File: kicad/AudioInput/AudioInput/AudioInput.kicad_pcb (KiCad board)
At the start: 2 copper layers, 48.9 x 55.5 mm, 61 parts, among them J1 EXPAN2, J2 EXPAN1, J3 INT INPUT, K1 G6K-2, Q1 BS250, Q2 2N7000, Q3 BS250, U1 MCP4651, U2 LM324, U3 CD4052B

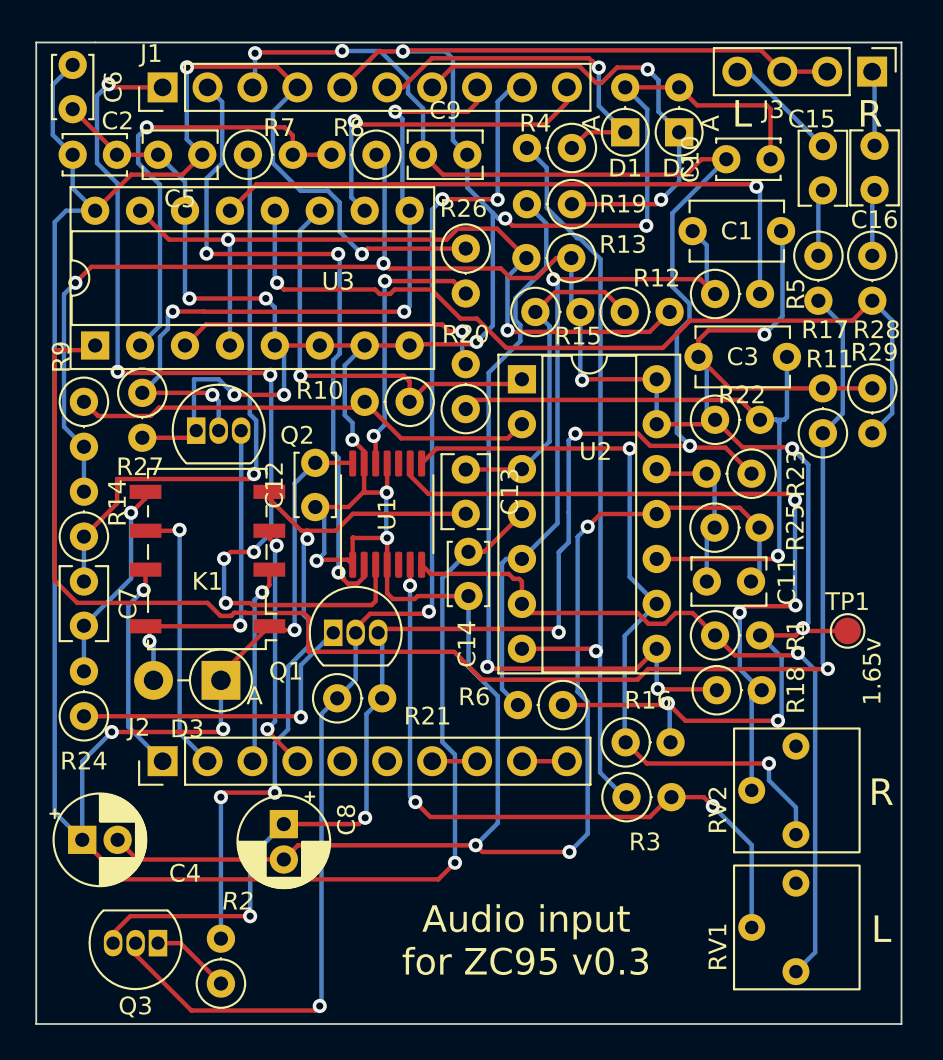
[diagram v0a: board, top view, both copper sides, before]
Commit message: Audio input board v0.4
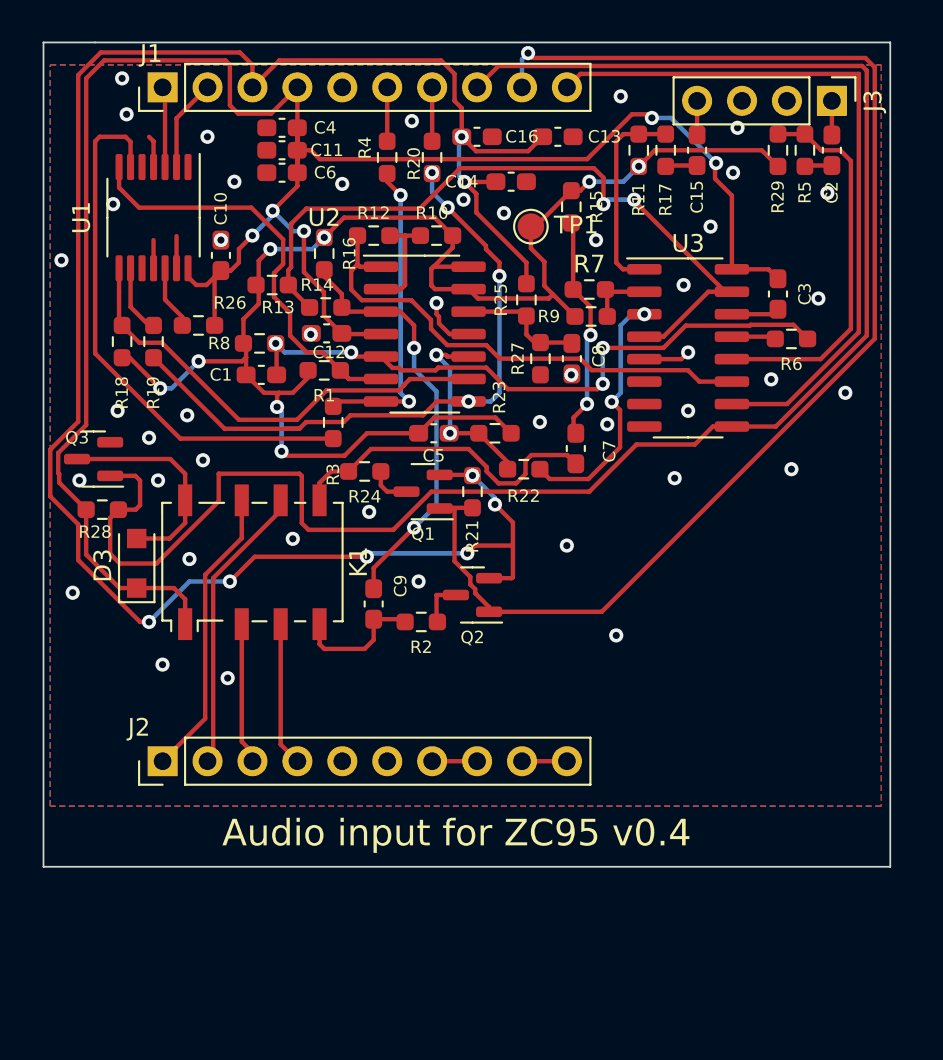
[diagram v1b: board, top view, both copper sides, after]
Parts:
- removed D1, D2: 3.3v, Diode_THT:D_DO-35_SOD27_P2.54mm_Vertical_AnodeUp
- removed RV1, RV2: 50k, Library:3362P-1-503
- C1: value 3nF -> 3.3nF; footprint Capacitor_THT:C_Disc_D5.1mm_W3.2mm_P5.00mm -> Capacitor_SMD:C_0603_1608Metric_Pad1.08x0.95mm_HandSolder
- C10, C12, C6: footprint Capacitor_THT:C_Disc_D3.4mm_W2.1mm_P2.50mm -> Capacitor_SMD:C_0603_1608Metric_Pad1.08x0.95mm_HandSolder
- C11, C15, C7, C9: footprint Capacitor_THT:C_Rect_L4.0mm_W2.5mm_P2.50mm -> Capacitor_SMD:C_0603_1608Metric_Pad1.08x0.95mm_HandSolder
- C13: value 1uF -> 10uF; footprint Capacitor_THT:C_Rect_L4.0mm_W2.5mm_P2.50mm -> Capacitor_SMD:C_0603_1608Metric_Pad1.08x0.95mm_HandSolder
- C14, C2: value 100nF -> 1uF; footprint Capacitor_THT:C_Disc_D3.4mm_W2.1mm_P2.50mm -> Capacitor_SMD:C_0603_1608Metric_Pad1.08x0.95mm_HandSolder
- C16: value 1uF -> 100nF; footprint Capacitor_THT:C_Rect_L4.0mm_W2.5mm_P2.50mm -> Capacitor_SMD:C_0603_1608Metric_Pad1.08x0.95mm_HandSolder
- C3: value 3nF -> 100nF; footprint Capacitor_THT:C_Disc_D5.1mm_W3.2mm_P5.00mm -> Capacitor_SMD:C_0603_1608Metric_Pad1.08x0.95mm_HandSolder
- C4: footprint Capacitor_THT:CP_Radial_D5.0mm_P2.00mm -> Capacitor_SMD:C_0603_1608Metric_Pad1.08x0.95mm_HandSolder
- C5: value 1uF -> 3.3nF; footprint Capacitor_THT:C_Rect_L4.0mm_W2.5mm_P2.50mm -> Capacitor_SMD:C_0603_1608Metric_Pad1.08x0.95mm_HandSolder
- C8: value 10uF -> 1uF; footprint Capacitor_THT:CP_Radial_D5.0mm_P2.00mm -> Capacitor_SMD:C_0603_1608Metric_Pad1.08x0.95mm_HandSolder
- D3: value 1N4004 -> SM4007PL; footprint Diode_THT:D_DO-41_SOD81_P3.81mm_Vertical_AnodeUp -> Diode_SMD:D_SOD-123F
- Q1: value BS250 -> AO3401A; footprint Package_TO_SOT_THT:TO-92_Inline -> Package_TO_SOT_SMD:SOT-23
- Q2: value 2N7000 -> AO3401A; footprint Package_TO_SOT_THT:TO-92_Inline -> Package_TO_SOT_SMD:SOT-23
- Q3: value BS250 -> AO3400A; footprint Package_TO_SOT_THT:TO-92_Inline -> Package_TO_SOT_SMD:SOT-23
- R1, R11, R12, R15, R17, R21, R23, R25, R26, R27, R28, R29, R3, R4, R7: footprint Resistor_THT:R_Axial_DIN0207_L6.3mm_D2.5mm_P2.54mm_Vertical -> Resistor_SMD:R_0603_1608Metric_Pad0.98x0.95mm_HandSolder
- R10: value 100k -> 4k7; footprint Resistor_THT:R_Axial_DIN0207_L6.3mm_D2.5mm_P2.54mm_Vertical -> Resistor_SMD:R_0603_1608Metric_Pad0.98x0.95mm_HandSolder
- R13, R8: value 150k -> 100k; footprint Resistor_THT:R_Axial_DIN0207_L6.3mm_D2.5mm_P2.54mm_Vertical -> Resistor_SMD:R_0603_1608Metric_Pad0.98x0.95mm_HandSolder
- R14: value 100k -> 150k; footprint Resistor_THT:R_Axial_DIN0207_L6.3mm_D2.5mm_P2.54mm_Vertical -> Resistor_SMD:R_0603_1608Metric_Pad0.98x0.95mm_HandSolder
- R16: value 4k7 -> 100k; footprint Resistor_THT:R_Axial_DIN0207_L6.3mm_D2.5mm_P2.54mm_Vertical -> Resistor_SMD:R_0603_1608Metric_Pad0.98x0.95mm_HandSolder
- R18: value 10k -> 4k7; footprint Resistor_THT:R_Axial_DIN0207_L6.3mm_D2.5mm_P2.54mm_Vertical -> Resistor_SMD:R_0603_1608Metric_Pad0.98x0.95mm_HandSolder
- R19: value 1k -> 10k; footprint Resistor_THT:R_Axial_DIN0207_L6.3mm_D2.5mm_P2.54mm_Vertical -> Resistor_SMD:R_0603_1608Metric_Pad0.98x0.95mm_HandSolder
- R2, R24: value 2k7 -> 2k2; footprint Resistor_THT:R_Axial_DIN0207_L6.3mm_D2.5mm_P2.54mm_Vertical -> Resistor_SMD:R_0603_1608Metric_Pad0.98x0.95mm_HandSolder
- R20: value 10k -> 1k; footprint Resistor_THT:R_Axial_DIN0207_L6.3mm_D2.5mm_P2.54mm_Vertical -> Resistor_SMD:R_0603_1608Metric_Pad0.98x0.95mm_HandSolder
- R22, R6: value 100k -> 10k; footprint Resistor_THT:R_Axial_DIN0207_L6.3mm_D2.5mm_P2.54mm_Vertical -> Resistor_SMD:R_0603_1608Metric_Pad0.98x0.95mm_HandSolder
- R5: value 10k -> 100k; footprint Resistor_THT:R_Axial_DIN0207_L6.3mm_D2.5mm_P2.54mm_Vertical -> Resistor_SMD:R_0603_1608Metric_Pad0.98x0.95mm_HandSolder
- R9: value 10k -> 150k; footprint Resistor_THT:R_Axial_DIN0207_L6.3mm_D2.5mm_P2.54mm_Vertical -> Resistor_SMD:R_0603_1608Metric_Pad0.98x0.95mm_HandSolder
- U2: footprint Package_DIP:DIP-14_W7.62mm_Socket -> Package_SO:SOIC-14_3.9x8.7mm_P1.27mm
- U3: footprint Package_DIP:DIP-16_W7.62mm_Socket -> Package_SO:SOIC-16_3.9x9.9mm_P1.27mm
- moved R28 45.8 mm to (132.5, 89.9), turned to 0 degrees
- moved C4 41.8 mm to (142.6, 68.3), turned to 180 degrees
- moved C2 40.4 mm to (173.7, 69.6), turned to -90 degrees
- moved R18 39.0 mm to (133.6, 80.4), turned to -90 degrees
- moved C11 36.0 mm to (142.6, 69.6), turned to 0 degrees
- moved U3 33.5 mm to (165.6, 80.8), turned to 0 degrees
- moved R16 32.5 mm to (145.0, 75.4), turned to -90 degrees
- moved C8 30.9 mm to (159.0, 81.4), turned to 90 degrees
- moved C10 29.1 mm to (139.2, 75.5), turned to 90 degrees
- moved R9 29.1 mm to (160.1, 79.0), turned to 0 degrees
- moved TP1 29.0 mm to (156.7, 73.9)
- moved C7 28.8 mm to (159.3, 86.5)
- moved Q3 27.6 mm to (132.0, 87.1)
- moved R3 26.9 mm to (145.5, 85.0), turned to -90 degrees
- moved R1 26.7 mm to (145.0, 82.0), turned to 180 degrees
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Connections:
- C10 pad 1: 3v3 -> 5v
- C11 pad 2: Net-(C11-Pad2) -> 5v
- C12 pad 1: GND -> 5v
- C12 pad 2: 5v -> GND
- C13 pad 1: AUDIO_IN_L -> 3v3
- C13 pad 2: Net-(C13-Pad2) -> GND
- C14 pad 2: 5v -> 3v3
- C16 pad 1: Net-(C16-Pad1) -> 3v3
- C16 pad 2: Net-(C16-Pad2) -> GND
- C2 pad 1: GND -> Net-(J3-Pad1)
- C2 pad 2: 5v -> Net-(C2-Pad2)
- C3 pad 1: Net-(C3-Pad1) -> GND
- C3 pad 2: 1.65v -> 5v
- C5 pad 1: 5v -> Net-(U2-Pad10)
- C5 pad 2: GND -> 1.65v
- C8 pad 1: 3v3 -> GND
- C8 pad 2: GND -> Net-(U2-Pad12)
- C9 pad 1: 3v3 -> AUDIO_IN_L
- C9 pad 2: GND -> Net-(K1-Pad4)
- D3 pad 2: Net-(K1-Pad8) -> Net-(D3-Pad2)
- J3 pad 1: Net-(C16-Pad1) -> Net-(J3-Pad1)
- K1 pad 4: Net-(C13-Pad2) -> Net-(K1-Pad4)
- K1 pad 8: Net-(K1-Pad8) -> Net-(D3-Pad2)
- Q1 pad 1: Net-(Q1-Pad1) -> MIC_PWR_DIS
- Q1 pad 2: MIC_PWR_DIS -> 3v3
- Q1 pad 3: 3v3 -> Net-(R24-Pad1)
- Q2 pad 1: GND -> MIC_PWR_DIS
- Q2 pad 2: AUDIO_EN -> 3v3
- Q2 pad 3: Net-(K1-Pad8) -> Net-(R2-Pad1)
- Q3 pad 1: Net-(Q3-Pad1) -> AUDIO_EN
- Q3 pad 2: MIC_PWR_DIS -> GND
- Q3 pad 3: 3v3 -> Net-(D3-Pad2)
- R10 pad 1: MIC_PREAMP_OUT -> Net-(U2-Pad2)
- R10 pad 2: Net-(R10-Pad2) -> 1.65v
- R12 pad 1: AUDIO_IN_L -> Net-(U2-Pad2)
- R12 pad 2: Net-(R12-Pad2) -> MIC_PREAMP_OUT
- R13 pad 1: 1.65v -> AUDIO_IN_L
- R13 pad 2: Net-(R12-Pad2) -> Net-(U3-Pad15)
- R14 pad 1: AUDIO_IN_R -> 1.65v
- R14 pad 2: 1.65v -> Net-(U3-Pad15)
- R15 pad 1: AUDIO_IN_L -> 1.65v
- R15 pad 2: 1.65v -> AUDIO_IN_R
- R16 pad 1: Net-(R16-Pad1) -> 1.65v
- R16 pad 2: 1.65v -> AUDIO_IN_L
- R18 pad 1: Net-(R18-Pad1) -> Net-(U1-Pad8)
- R18 pad 2: Net-(R18-Pad2) -> 1.65v
- R19 pad 1: ADC2 -> Net-(U2-Pad8)
- R19 pad 2: Net-(R18-Pad1) -> Net-(U1-Pad9)
- R2 pad 1: Net-(Q3-Pad1) -> Net-(R2-Pad1)
- R2 pad 2: Net-(C13-Pad2) -> Net-(K1-Pad4)
- R20 pad 1: Net-(C3-Pad1) -> ADC2
- R20 pad 2: AUDIO_R -> Net-(U2-Pad8)
- R22 pad 1: 1.65v -> Net-(U2-Pad10)
- R22 pad 2: Net-(C3-Pad1) -> AUDIO_R
- R23 pad 1: 3v3 -> 1.65v
- R23 pad 2: Net-(C11-Pad2) -> Net-(U2-Pad10)
- R24 pad 1: Net-(Q1-Pad1) -> Net-(R24-Pad1)
- R25 pad 1: Net-(C11-Pad2) -> Net-(U2-Pad12)
- R25 pad 2: GND -> 3v3
- R27 pad 1: AUDIO_EN -> Net-(U2-Pad12)
- R28 pad 1: Net-(C16-Pad2) -> 5v
- R28 pad 2: INT_INPUT_R -> AUDIO_EN
- R5 pad 1: Net-(C1-Pad1) -> Net-(C2-Pad2)
- R5 pad 2: AUDIO_L -> INT_INPUT_R
- R6 pad 1: 1.65v -> Net-(C1-Pad1)
- R6 pad 2: Net-(C1-Pad1) -> AUDIO_L
- R7 pad 2: Net-(R7-Pad2) -> Net-(R9-Pad2)
- R8 pad 2: Net-(R7-Pad2) -> Net-(C1-Pad1)
- R9 pad 1: Net-(R10-Pad2) -> 1.65v
- R9 pad 2: 1.65v -> Net-(R9-Pad2)
- U1 pad 8: Net-(R16-Pad1) -> Net-(U1-Pad8)
- U1 pad 9: Net-(R18-Pad2) -> Net-(U1-Pad9)
- U2 pad 10: Net-(C3-Pad1) -> Net-(U2-Pad10)
- U2 pad 12: Net-(C11-Pad2) -> Net-(U2-Pad12)
- U2 pad 2: Net-(R10-Pad2) -> Net-(U2-Pad2)
- U2 pad 8: Net-(R18-Pad1) -> Net-(U2-Pad8)
- U2 pad 9: Net-(R16-Pad1) -> Net-(U1-Pad8)
- U3 pad 15: Net-(R12-Pad2) -> Net-(U3-Pad15)
- U3 pad 2: Net-(R7-Pad2) -> Net-(R9-Pad2)
- U3 pad 4: Net-(R12-Pad2) -> Net-(U3-Pad15)
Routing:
- net GND: track 236.1 -> 13.7 mm, vias 15 -> 45
- net INT_INPUT_L: track 84.9 -> 11.6 mm, vias 1 -> 0
- net AUDIO_EN: track 42.1 -> 98.3 mm, vias 4 -> 0
- net SDA: track 54.6 -> 4.56 mm, vias 6 -> 0
- net 1.65v: track 132.6 -> 85.9 mm
- net 5v: track 164.8 -> 119.0 mm, vias 6 -> 5
- net Net-(R18-Pad1): track 43.8 -> 0.00 mm, vias 2 -> 0
- net Net-(R18-Pad2): track 43.7 -> 0.00 mm, vias 3 -> 0
- net Net-(R12-Pad2): track 43.7 -> 0.00 mm, vias 2 -> 0
- net Net-(R16-Pad1): track 43.4 -> 0.00 mm, vias 2 -> 0
- net Net-(U3-Pad15): track 0.00 -> 41.7 mm, vias 0 -> 2
- net Net-(C13-Pad2): track 39.6 -> 0.00 mm, vias 3 -> 0
- net Net-(C3-Pad1): track 38.0 -> 0.00 mm, vias 1 -> 0
- net Net-(U2-Pad8): track 0.00 -> 36.9 mm, vias 0 -> 4
- net AUDIO_L: track 36.6 -> 2.51 mm, vias 1 -> 0
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- added copper zone on B.Cu, net GND
- added copper zone on F.Cu, net GND
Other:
- board size 48.9 x 55.5 mm -> 47.9 x 46.6 mm
- board text added: "Audio input for ZC95 v0.4"
- board text removed: "1.65v"
- board text removed: "Audio input for ZC95 v0.3"
- board text removed: "L"
- board text removed: "R"
